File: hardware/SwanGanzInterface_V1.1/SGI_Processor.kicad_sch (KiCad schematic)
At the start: 22 parts, among them J2 Conn_01x08_Pin, SW2 MODE, SW3 ENTER, U4 XM0G3507QPTRQ1, U5 AdaFruit_1590, U7 FT232R

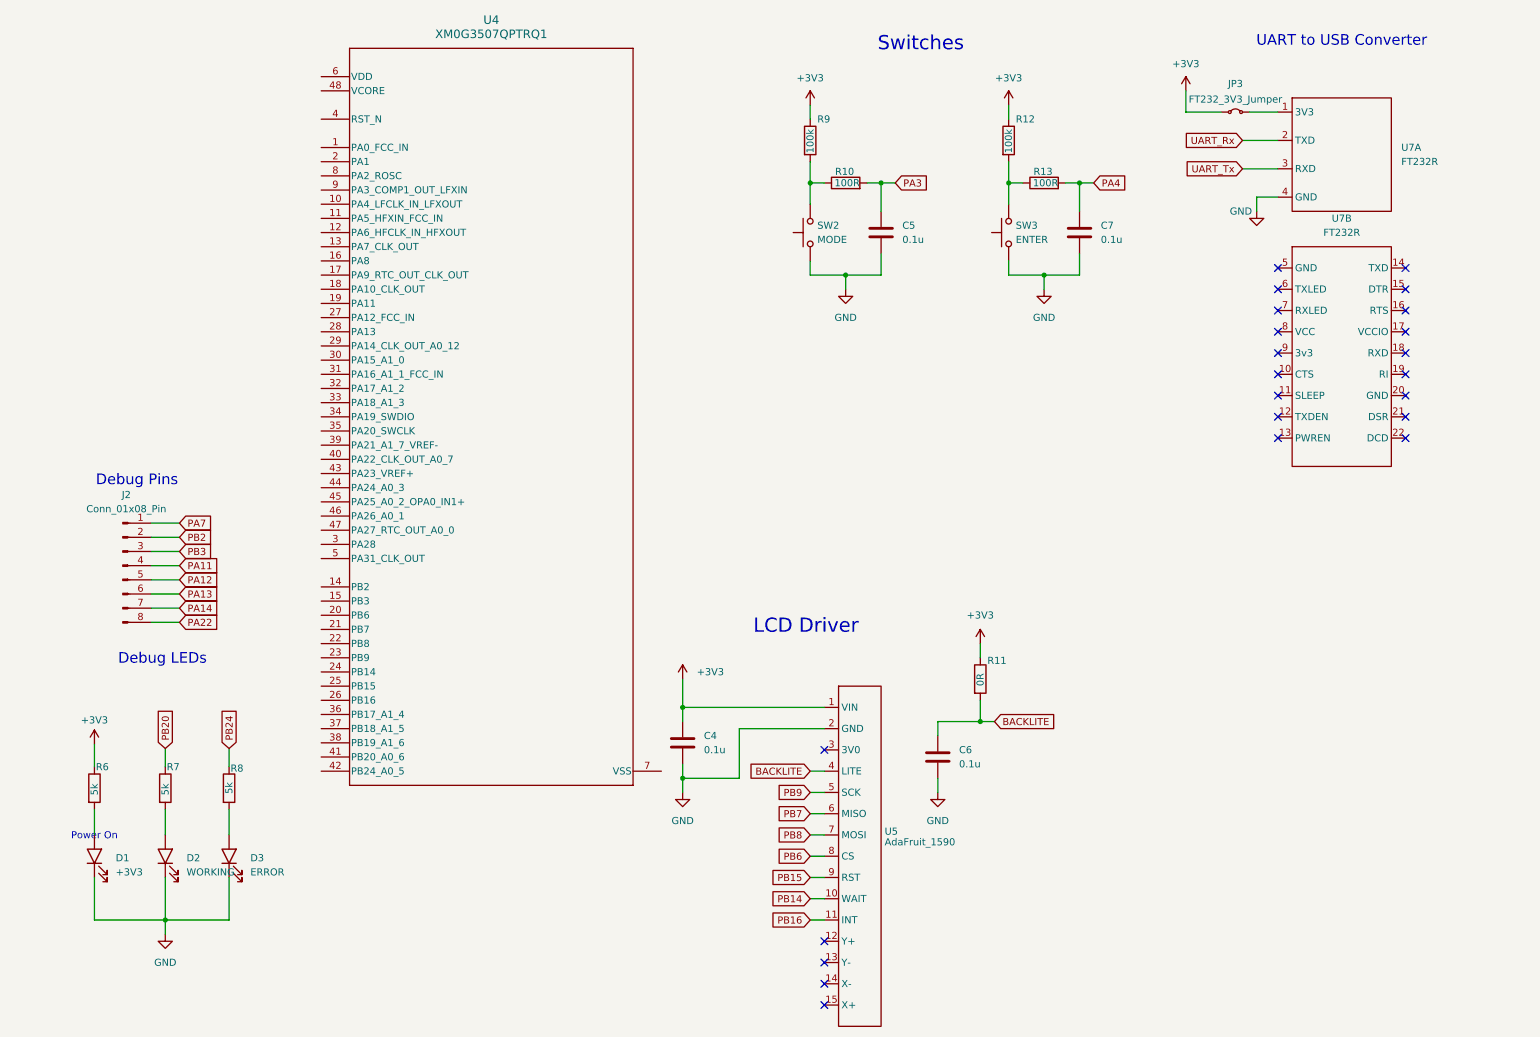
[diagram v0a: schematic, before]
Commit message: Hooked up MSP
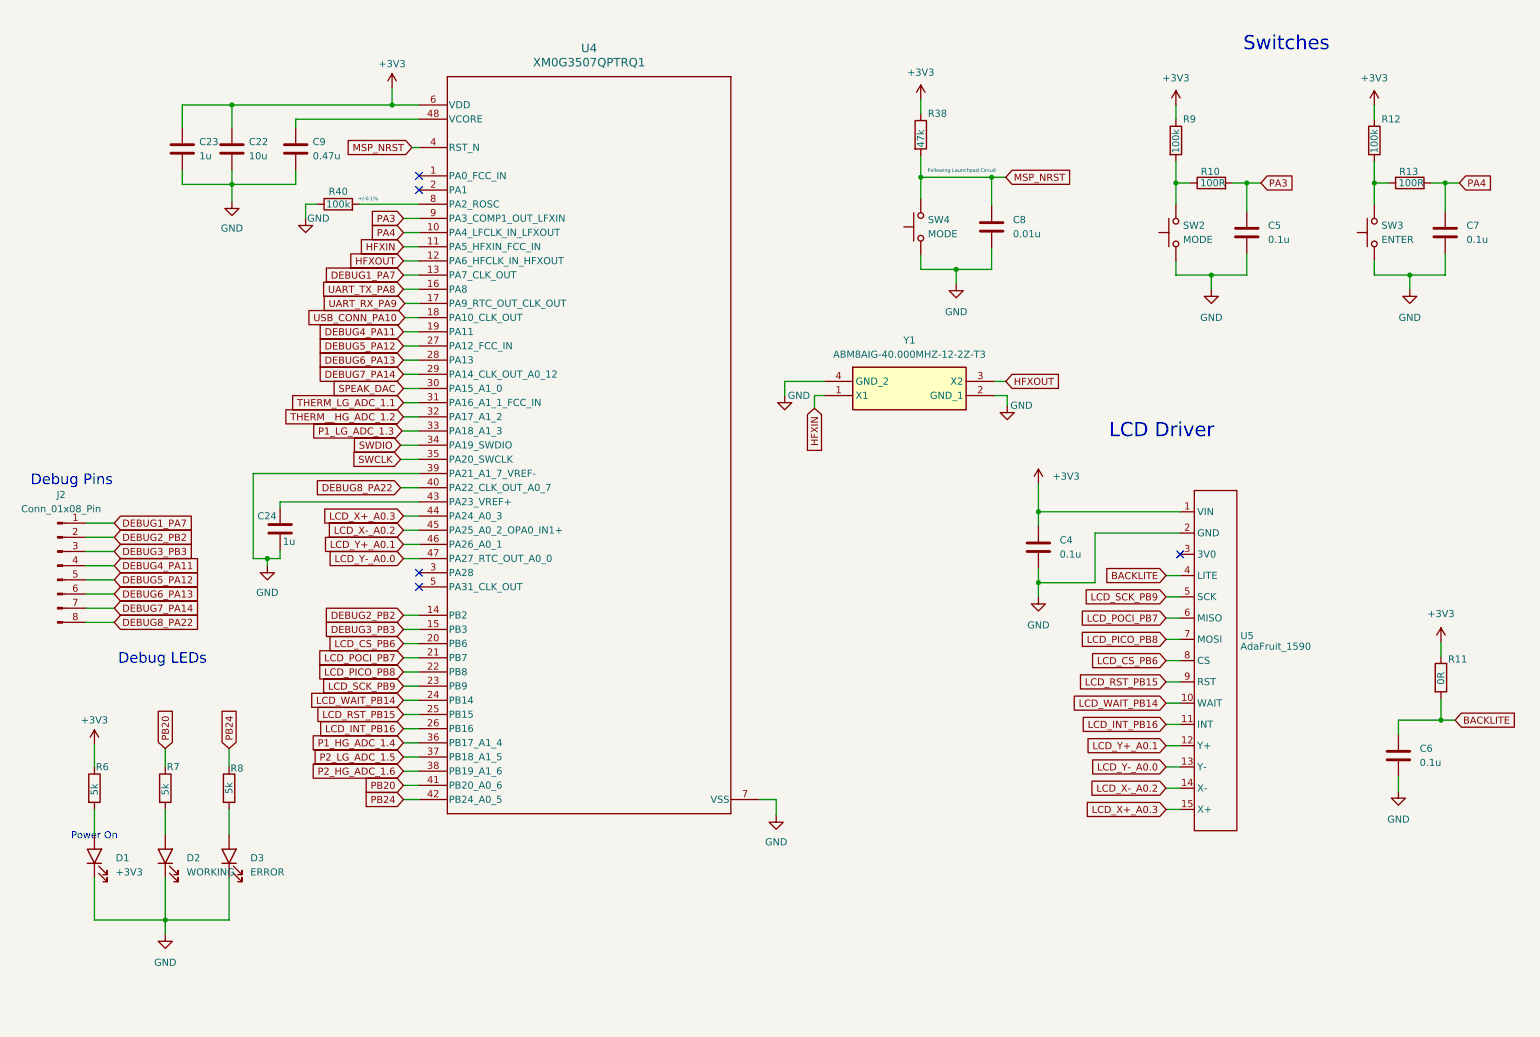
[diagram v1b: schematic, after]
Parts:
- removed JP3: FT232_3V3_Jumper, SGI_FootprintsLib:PinHeader_1x02_P2.54mm_Vertical, symbol Jumper:Jumper_2_Small_Bridged
- removed U7: FT232R, SGI_FootprintsLib:FT232R-Breakout, symbol SGI_SymbolLib:FT232R-Breakout
- added C22: 10u, symbol Device:C
- added C23, C24: 1u, symbol Device:C
- added C8: 0.01u, Capacitor_SMD:C_0603_1608Metric, symbol Device:C
- added C9: 0.47u, symbol Device:C
- added R38: 47k, Resistor_SMD:R_0603_1608Metric, symbol Device:R
- added R40: 100k, symbol Device:R
- added SW4: MODE, SGI_FootprintsLib:SW_PUSH_6mm, symbol SGI_SymbolLib:SW_Push
- added Y1: ABM8AIG-40.000MHZ-12-2Z-T3, SGI_FootprintsLib:ABM8AIG25000MHZ122ZT3, symbol SGI_SymbolLib:ABM8AIG-40.000MHZ-12-2Z-T3
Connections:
- net PA11 is gone; now on net DEBUG4_PA11: J2.4 (Pin_4)
- net PA12 is gone; now on net DEBUG5_PA12: J2.5 (Pin_5)
- net PA13 is gone; now on net DEBUG6_PA13: J2.6 (Pin_6)
- net PA14 is gone; now on net DEBUG7_PA14: J2.7 (Pin_7)
- net PA22 is gone; now on net DEBUG8_PA22: J2.8 (Pin_8)
- net PA7 is gone; now on net DEBUG1_PA7: J2.1 (Pin_1)
- net PB14 is gone; now on net LCD_WAIT_PB14: U5.10 (WAIT)
- net PB15 is gone; now on net LCD_RST_PB15: U5.9 (RST)
- net PB16 is gone; now on net LCD_INT_PB16: U5.11 (INT)
- net PB2 is gone; now on net DEBUG2_PB2: J2.2 (Pin_2)
- net PB3 is gone; now on net DEBUG3_PB3: J2.3 (Pin_3)
- net PB6 is gone; now on net LCD_CS_PB6: U5.8 (CS)
- net PB7 is gone; now on net LCD_POCI_PB7: U5.6 (MISO)
- net PB8 is gone; now on net LCD_PICO_PB8: U5.7 (MOSI)
- net PB9 is gone; now on net LCD_SCK_PB9: U5.5 (SCK)
- net +3V3: now also U4.6 (VDD), C22.1, C23.1, R38.1
- net GND: now also U4.39 (PA21_A1_7_VREF-), U4.7 (VSS), C22.2, C23.2, C24.2, C8.2, C9.2, R40.1, SW4.1, Y1.2 (GND_1), Y1.4 (GND_2)
- net PA3: now also U4.9 (PA3_COMP1_OUT_LFXIN)
- net PA4: now also U4.10 (PA4_LFCLK_IN_LFXOUT)
- net PB20: now also U4.41 (PB20_A0_6)
- net PB24: now also U4.42 (PB24_A0_5)
- net LCD_Y+_A0.1: now reaches U5.12 (Y+)
- net LCD_Y+_A0.1: now also U4.46 (PA26_A0_1)
- net LCD_Y-_A0.0: now reaches U5.13 (Y-)
- net LCD_Y-_A0.0: now also U4.47 (PA27_RTC_OUT_A0_0)
- net LCD_X-_A0.2: now reaches U5.14 (X-)
- net LCD_X-_A0.2: now also U4.45 (PA25_A0_2_OPA0_IN1+)
- net LCD_X+_A0.3: now reaches U5.15 (X+)
- net LCD_X+_A0.3: now also U4.44 (PA24_A0_3)
- net HFXIN: now reaches U4.11 (PA5_HFXIN_FCC_IN)
- net HFXIN: now also Y1.1 (X1)
- net HFXOUT: now reaches U4.12 (PA6_HFCLK_IN_HFXOUT)
- net HFXOUT: now also Y1.3 (X2)
- net DEBUG1_PA7: now reaches U4.13 (PA7_CLK_OUT)
- net DEBUG2_PB2: now reaches U4.14 (PB2)
- net DEBUG3_PB3: now reaches U4.15 (PB3)
- net UART_TX_PA8: now reaches U4.16 (PA8)
- net UART_RX_PA9: now reaches U4.17 (PA9_RTC_OUT_CLK_OUT)
- net USB_CONN_PA10: now reaches U4.18 (PA10_CLK_OUT)
- net DEBUG4_PA11: now reaches U4.19 (PA11)
- net LCD_CS_PB6: now reaches U4.20 (PB6)
- net LCD_POCI_PB7: now reaches U4.21 (PB7)
- net LCD_PICO_PB8: now reaches U4.22 (PB8)
- net LCD_SCK_PB9: now reaches U4.23 (PB9)
- net LCD_WAIT_PB14: now reaches U4.24 (PB14)
- net LCD_RST_PB15: now reaches U4.25 (PB15)
- net LCD_INT_PB16: now reaches U4.26 (PB16)
- net DEBUG5_PA12: now reaches U4.27 (PA12_FCC_IN)
- net DEBUG6_PA13: now reaches U4.28 (PA13)
- net DEBUG7_PA14: now reaches U4.29 (PA14_CLK_OUT_A0_12)
- net SPEAK_DAC: now reaches U4.30 (PA15_A1_0)
- net THERM_LG_ADC_1.1: now reaches U4.31 (PA16_A1_1_FCC_IN)
- net THERM__HG_ADC_1.2: now reaches U4.32 (PA17_A1_2)
- net P1_LG_ADC_1.3: now reaches U4.33 (PA18_A1_3)
- net SWDIO: now reaches U4.34 (PA19_SWDIO)
- net SWCLK: now reaches U4.35 (PA20_SWCLK)
- net P1_HG_ADC_1.4: now reaches U4.36 (PB17_A1_4)
- net P2_LG_ADC_1.5: now reaches U4.37 (PB18_A1_5)
- net P2_HG_ADC_1.6: now reaches U4.38 (PB19_A1_6)
- net MSP_NRST: now reaches U4.4 (RST_N)
- net MSP_NRST: now also C8.1, R38.2, SW4.2
- net DEBUG8_PA22: now reaches U4.40 (PA22_CLK_OUT_A0_7)
- net at U4.43 (PA23_VREF+): now also C24.1
- net at U4.48 (VCORE): now also C9.1
- net at U4.8 (PA2_ROSC): now also R40.2
- no-connect marks 23 -> 5
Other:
- note added: "+/-0.1%"
- note added: "Following Launchpad Circuit"
- note removed: "UART to USB Converter"
- moved on the sheet: C4, C5, C6, C7, J2, R10, R11, R12, R13, R9, SW2, SW3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
